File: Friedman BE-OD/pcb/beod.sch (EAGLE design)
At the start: 64 parts, among them IC1 TL072, IC2 TL072, IC3 TL062, J1 POWER_JACK, X1 2510-

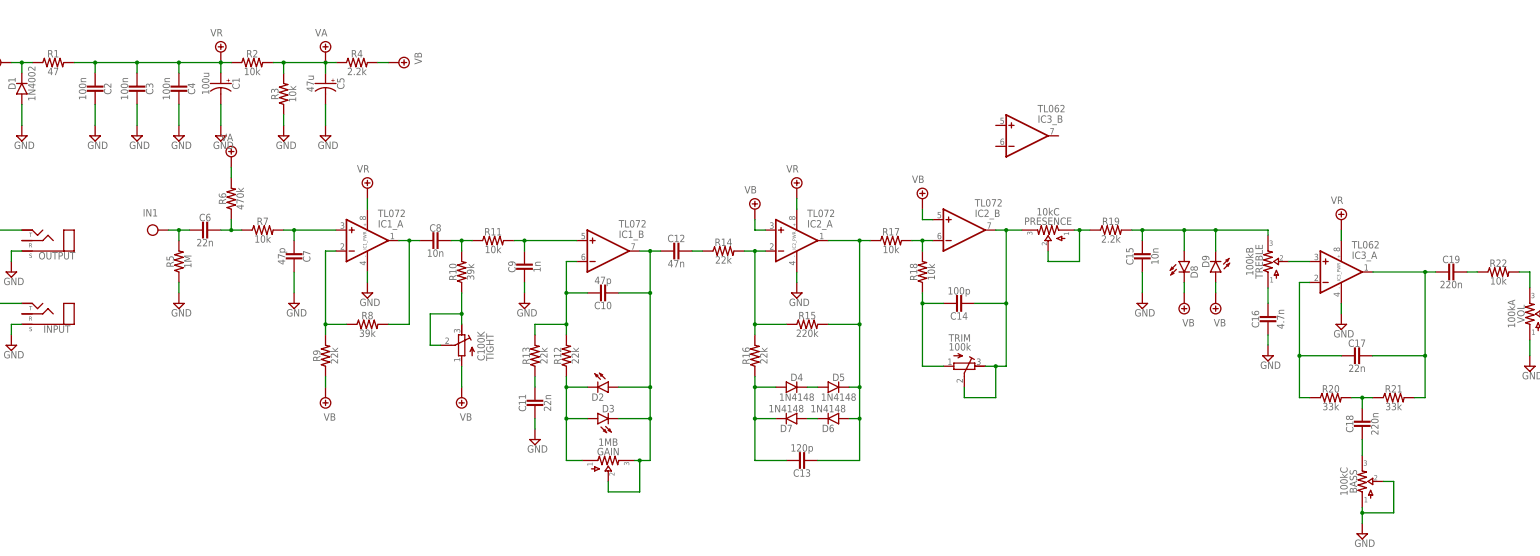
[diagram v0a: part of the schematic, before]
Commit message: 20180529
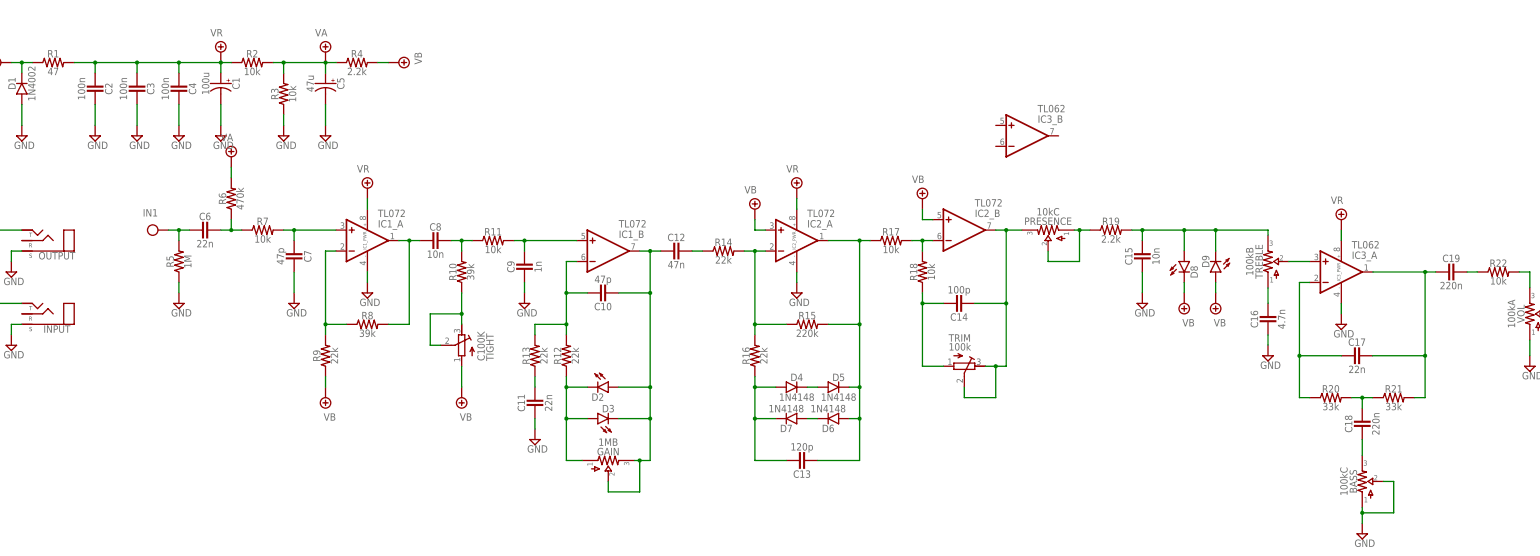
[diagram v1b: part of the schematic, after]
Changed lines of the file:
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@@
 <?xml version="1.0" encoding="utf-8"?>
 <!DOCTYPE eagle SYSTEM "eagle.dtd">
-<eagle version="7.6.0">
+<eagle version="8.5.1">
 <drawing>
 <settings>
 <setting alwaysvectorfont="no"/>
+<setting keepoldvectorfont="yes"/>
 <setting verticaltext="up"/>
 </settings>
@@
 <layer number="59" name="tCarbon" color="7" fill="1" visible="no" active="no"/>
 <layer number="60" name="bCarbon" color="7" fill="1" visible="no" active="no"/>
+<layer number="88" name="SimResults" color="9" fill="1" visible="yes" active="yes"/>
+<layer number="89" name="SimProbes" color="9" fill="1" visible="yes" active="yes"/>
 <layer number="90" name="Modules" color="5" fill="1" visible="yes" active="yes"/>
 <layer number="91" name="Nets" color="2" fill="1" visible="yes" active="yes"/>
